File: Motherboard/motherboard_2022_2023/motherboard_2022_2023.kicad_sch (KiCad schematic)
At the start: 31 parts, among them J1 Conn_01x02_Female, J10 Conn_01x03_Male, J2 Raspberry_Pi_2_3, J3 Conn_01x03_Male, J4 Conn_01x03_Male, J5 Conn_01x03_Male, J6 Conn_01x03_Male, J7 Conn_01x03_Male, J8 Conn_01x03_Male, J9 Conn_01x03_Male, U1 XBee_THT, U2 MPU-6050-Breakout, U3 PCA9685PW, U4 MPL3115A2, U6 SAM-M8Q, U7 MPU-6050

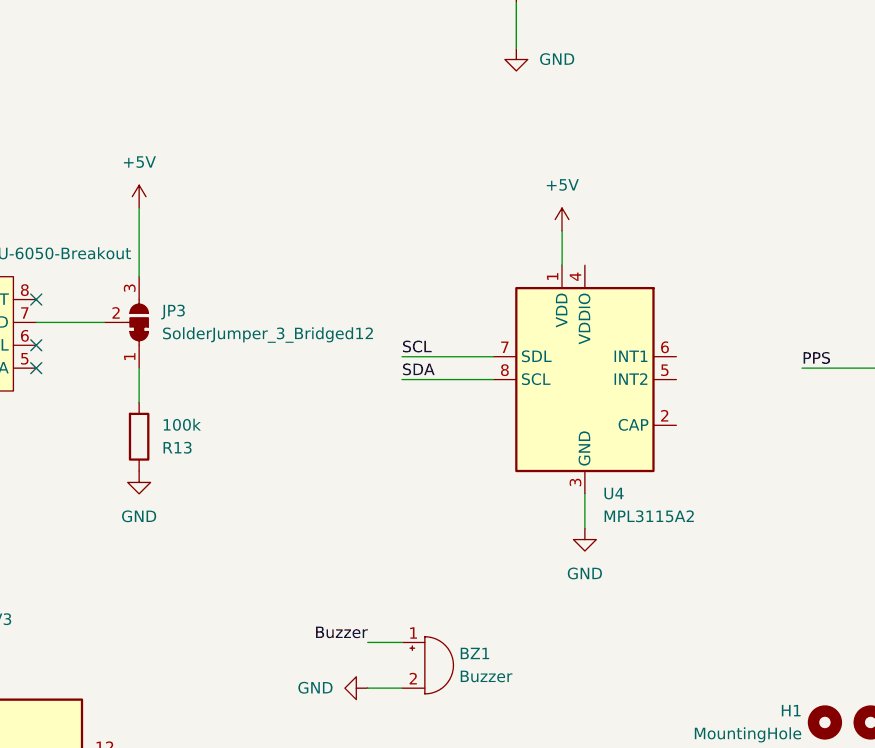
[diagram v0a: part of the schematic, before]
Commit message: Add capacitors to MPL3115 according to the datasheet
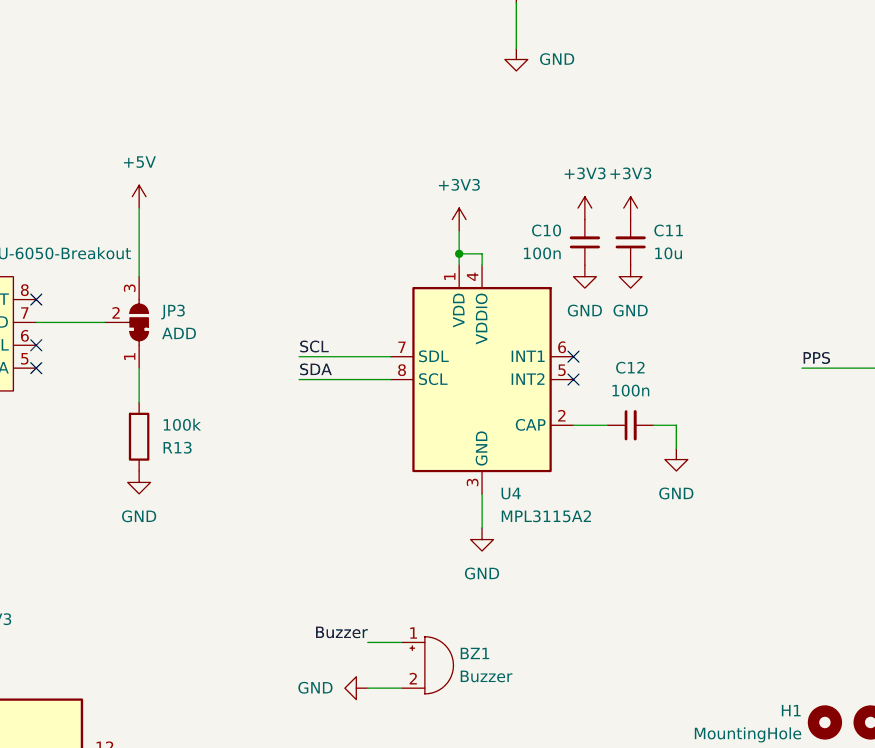
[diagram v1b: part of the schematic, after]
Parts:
- added C10, C12: 100n, Capacitor_SMD:C_0603_1608Metric, symbol Device:C_Small
- added C11: 10u, Capacitor_SMD:C_0603_1608Metric, symbol Device:C_Small
- JP3: value SolderJumper_3_Bridged12 -> ADD
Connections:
- net +3V3: now also U4.1 (VDD), U4.4 (VDDIO), C10.2, C11.2
- net +5V: no longer U4.1 (VDD)
- net GND: now also C10.1, C11.1, C12.2
- net at U4.2 (CAP): now also C12.1
- no-connect marks 16 -> 18
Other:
- moved on the sheet: U4
